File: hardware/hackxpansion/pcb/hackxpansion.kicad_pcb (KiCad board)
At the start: 4 copper layers, 52 x 69 mm, 101 parts, among them CN1 533981471, CN2 533981471, CN3 533981471, CN4 533981471, IC1 ADS7128IRTET, J1 Conn_01x03_MountingPin, J2 USB_C_Receptacle_USB2.0_14P, Q1 BSS138, Q2 2N7002, SW1 SW_Push, SW2 SW_Push, SW3 SW_On_Off, U2 RP2354B, U5 SPX3819M5-L-3-3, U7 BQ24075RGT, U8 USBLC6-2SC6, Y1 ABM8-272-T3

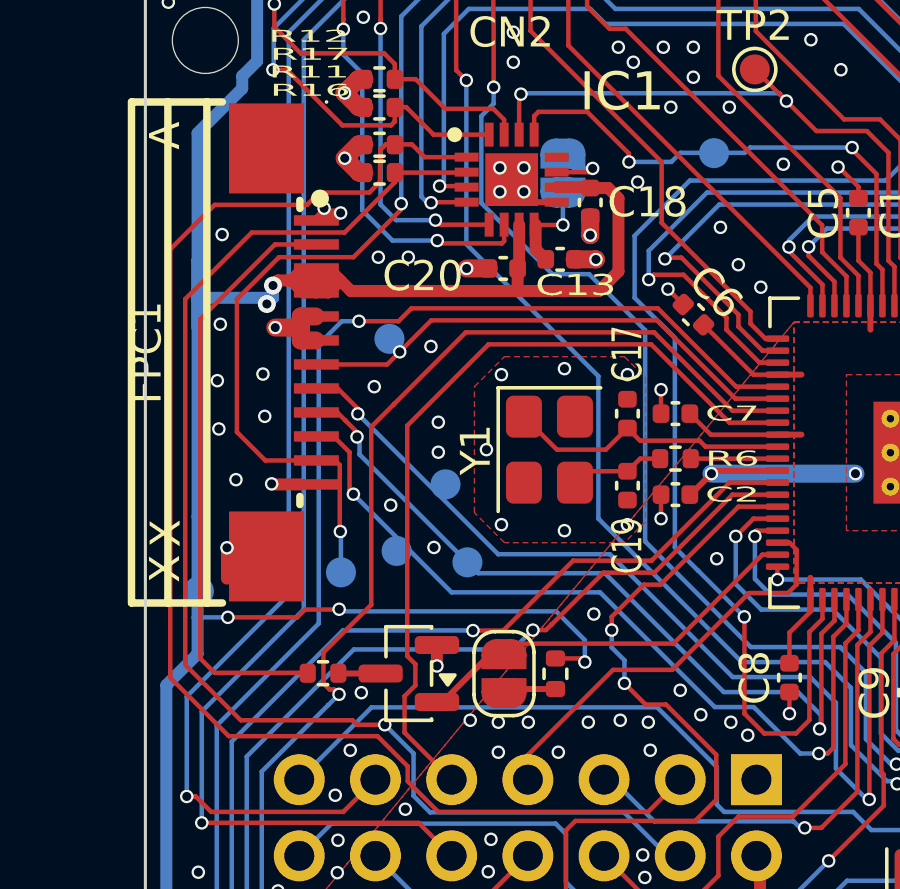
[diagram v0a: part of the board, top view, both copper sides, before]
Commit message: fixed issues with new fpc
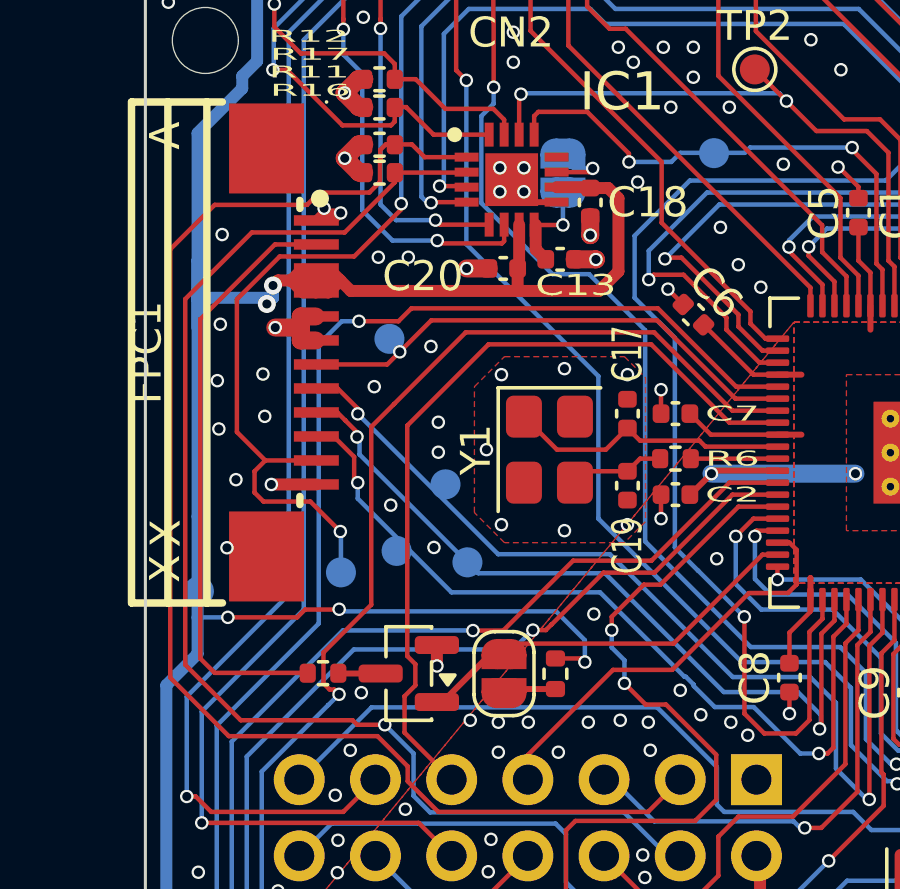
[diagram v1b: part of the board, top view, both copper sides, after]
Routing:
- net /GND: track 62.5 -> 64.4 mm
- net /Main Board/Display/RESET: track 59.8 -> 61.0 mm
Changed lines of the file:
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@@
 		(capping no)
 		(filling no)
-		(zone_defaults)
 		(grid_origin 122.239998 40.72)
 		(pcbplotparams
@@
 	)
 	(segment
+		(start 105.62 81.81)
+		(end 105.91 82.1)
+		(width 0.4)
+		(layer "F.Cu")
+		(net "/GND")
+	)
+	(segment
 		(start 147.610459 96.500266)
 		(end 148.149423 96.500266)
@@
 	)
 	(segment
+		(start 104.59 81.81)
+		(end 105.62 81.81)
+		(width 0.4)
+		(layer "F.Cu")
+		(net "/GND")
+	)
+	(segment
 		(start 114.83 70.29)
 		(end 114.08 69.54)
@@
 	)
 	(segment
-		(start 104.59 82.840001)
-		(end 104.59 81.81)
-		(width 0.4)
-		(layer "F.Cu")
-		(net "/GND")
-	)
-	(segment
 		(start 107.827121 70.622879)
 		(end 107.55 70.9)
@@
 	)
 	(segment
+		(start 107.57 79.7)
+		(end 106.069998 79.7)
+		(width 0.4)
+		(layer "F.Cu")
+		(net "/GND")
+	)
+	(segment
 		(start 127.244998 93.277787)
 		(end 127.244998 92.65)
@@
 	)
 	(via
+		(at 106.069998 79.7)
+		(size 0.45)
+		(drill 0.3)
+		(layers "F.Cu" "B.Cu")
+		(net "/GND")
+	)
+	(via
 		(at 136.2 97.06)
 		(size 0.45)
@@
 	)
 	(via
-		(at 106.08 79.68)
-		(size 0.45)
-		(drill 0.3)
-		(layers "F.Cu" "B.Cu")
-		(free yes)
-		(net "/GND")
-	)
-	(via
 		(at 103.635738 92.625706)
 		(size 0.45)
@@
 	)
 	(segment
-		(start 108.676572 79.89654)
-		(end 108.676572 78.626572)
-		(width 0.15)
-		(layer "F.Cu")
-		(net "/Main Board/Display/MOSI")
-	)
-	(segment
 		(start 124.32 88.668245)
 		(end 124.61 88.668245)
@@
 	)
 	(segment
-		(start 108.676572 78.626572)
+		(start 108.829998 78.779998)
 		(end 108.16 78.11)
 		(width 0.15)
@@
 	)
 	(segment
-		(start 107.559999 78.11)
-		(end 107.549999 78.1)
+		(start 108.829998 79.519995)
+		(end 108.829998 78.779998)
 		(width 0.15)
 		(layer "F.Cu")
@@
 	)
 	(segment
+		(start 107.559999 78.11)
+		(end 107.549999 78.1)
+		(width 0.15)
+		(layer "F.Cu")
+		(net "/Main Board/Display/MOSI")
+	)
+	(segment
 		(start 108.16 78.11)
 		(end 107.559999 78.11)
@@
 	)
 	(segment
-		(start 108.805016 80.024984)
-		(end 108.676572 79.89654)
+		(start 108.950003 79.64)
+		(end 108.829998 79.519995)
 		(width 0.15)
 		(layer "F.Cu")
@@
 	)
 	(via
-		(at 108.805016 80.024984)
+		(at 108.950003 79.64)
 		(size 0.45)
 		(drill 0.3)
@@
 	)
 	(segment
-		(start 120.85 87.12)
-		(end 122.15 87.12)
+		(start 122.15 87.12)
+		(end 123.698245 88.668245)
 		(width 0.15)
 		(layer "B.Cu")
@@
 	)
 	(segment
-		(start 112.075032 83.295)
-		(end 117.025 83.295)
+		(start 108.950003 80.169971)
+		(end 112.075032 83.295)
 		(width 0.15)
 		(layer "B.Cu")
@@
 	)
 	(segment
-		(start 122.15 87.12)
-		(end 123.698245 88.668245)
+		(start 108.950003 79.64)
+		(end 108.950003 80.169971)
 		(width 0.15)
 		(layer "B.Cu")
@@
 	)
 	(segment
-		(start 108.805016 80.024984)
-		(end 112.075032 83.295)
+		(start 120.85 87.12)
+		(end 122.15 87.12)
+		(width 0.15)
+		(layer "B.Cu")
+		(net "/Main Board/Display/MOSI")
+	)
+	(segment
+		(start 120.15 86.373603)
+		(end 120.15 86.42)
 		(width 0.15)
 		(layer "B.Cu")
@@
 	)
 	(segment
+		(start 119.886397 86.11)
+		(end 120.15 86.373603)
+		(width 0.15)
+		(layer "B.Cu")
+		(net "/Main Board/Display/MOSI")
+	)
+	(segment
 		(start 117.025 83.295)
+		(end 119.84 86.11)
+		(width 0.15)
+		(layer "B.Cu")
+		(net "/Main Board/Display/MOSI")
+	)
+	(segment
+		(start 119.84 86.11)
+		(end 119.886397 86.11)
+		(width 0.15)
+		(layer "B.Cu")
+		(net "/Main Board/Display/MOSI")
+	)
+	(segment
+		(start 120.15 86.42)
 		(end 120.85 87.12)
 		(width 0.15)
@@
 	)
 	(segment
-		(start 110.4 70.53)
-		(end 108.805 72.125)
+		(start 112.075032 83.295)
+		(end 117.025 83.295)
+		(width 0.15)
+		(layer "B.Cu")
+		(net "/Main Board/Display/MOSI")
+	)
+	(segment
+		(start 104.921117 77.951117)
+		(end 105.87 78.9)
 		(width 0.15)
 		(layer "F.Cu")
@@
 	)
 	(segment
-		(start 108.805 72.125)
-		(end 106.324999 72.125)
+		(start 107.37 80.27)
+		(end 105.809998 80.27)
 		(width 0.15)
 		(layer "F.Cu")
@@
 	)
 	(segment
-		(start 107.05 79.7)
-		(end 106.1 79.7)
-		(width 0.4)
+		(start 105.509998 79.97)
+		(end 105.509998 79.260002)
+		(width 0.15)
 		(layer "F.Cu")
 		(net "/Main Board/Display/RESET")
 	)
 	(segment
-		(start 131.890003 67.91)
-		(end 131.840001 67.960002)
+		(start 108.83 72.1)
+		(end 106.349999 72.1)
 		(width 0.15)
 		(layer "F.Cu")
@@
 	)
 	(segment
-		(start 105.87 78.9)
-		(end 107.05 78.9)
+		(start 105.509998 79.260002)
+		(end 105.87 78.9)
 		(width 0.15)
 		(layer "F.Cu")
@@
 	)
 	(segment
-		(start 131.840001 67.960002)
-		(end 131.840001 72.34)
+		(start 110.4 70.34)
+		(end 110.4 70.53)
 		(width 0.15)
 		(layer "F.Cu")
@@
 	)
 	(segment
-		(start 108.35 81.25)
-		(end 108.35 79.05)
+		(start 131.890003 67.91)
+		(end 131.840001 67.960002)
 		(width 0.15)
 		(layer "F.Cu")
@@
 	)
 	(segment
-		(start 104.921117 73.528882)
-		(end 104.921117 77.951117)
+		(start 105.87 78.9)
+		(end 107.05 78.9)
 		(width 0.15)
 		(layer "F.Cu")
@@
 	)
 	(segment
-		(start 108.35 79.05)
-		(end 108.2 78.9)
+		(start 131.840001 67.960002)
+		(end 131.840001 72.34)
 		(width 0.15)
 		(layer "F.Cu")
@@
 	)
 	(segment
-		(start 106.324999 72.125)
-		(end 104.921117 73.528882)
+		(start 105.809998 80.27)
+		(end 105.509998 79.97)
 		(width 0.15)
 		(layer "F.Cu")
@@
 	)
 	(segment
-		(start 131.840001 72.34)
-		(end 131.240001 72.94)
+		(start 106.349999 72.1)
+		(end 104.921117 73.528882)
 		(width 0.15)
 		(layer "F.Cu")
@@
 	)
 	(segment
-		(start 106.1 79.7)
-		(end 106.08 79.68)
+		(start 131.840001 72.34)
+		(end 131.240001 72.94)
 		(width 0.15)
 		(layer "F.Cu")
@@
 	)
 	(segment
-		(start 104.921117 77.951117)
-		(end 105.87 78.9)
+		(start 110.4 70.53)
+		(end 108.83 72.1)
 		(width 0.15)
 		(layer "F.Cu")
@@
 	)
 	(segment
-		(start 131.240001 72.94)
-		(end 131.240002 73.743499)
+		(start 108.37 81.27)
+		(end 107.37 80.27)
 		(width 0.15)
 		(layer "F.Cu")
@@
 	)
 	(segment
-		(start 107.8 78.9)
-		(end 107.05 78.9)
+		(start 104.921117 73.528882)
+		(end 104.921117 77.951117)
 		(width 0.15)
 		(layer "F.Cu")
@@
 	)
 	(segment
-		(start 108.37 81.27)
-		(end 108.35 81.25)
+		(start 131.240001 72.94)
+		(end 131.240002 73.743499)
 		(width 0.15)
 		(layer "F.Cu")
@@
 	)
 	(segment
-		(start 110.4 70.34)
-		(end 110.4 70.53)
+		(start 107.8 78.9)
+		(end 107.05 78.9)
 		(width 0.15)
 		(layer "F.Cu")
@@
 	)
 	(segment
-		(start 108.511644 71.301644)
-		(end 110.18677 69.626519)
+		(start 105.42 71.3)
+		(end 108.513289 71.3)
 		(width 0.15)
 		(layer "F.Cu")
@@
 	)
 	(segment
-		(start 103.2 85.710001)
-		(end 103.2 73.52)
+		(start 108.93 87.710001)
+		(end 108.78 87.560001)
 		(width 0.15)
 		(layer "F.Cu")
@@
 	)
 	(segment
-		(start 110.185591 69.304687)
-		(end 112.565313 69.304687)
+		(start 108.78 87.560001)
+		(end 105.05 87.560001)
 		(width 0.15)
 		(layer "F.Cu")
@@
 	)
 	(segment
-		(start 105.05 87.560001)
-		(end 103.2 85.710001)
+		(start 110.185591 69.304687)
+		(end 112.565313 69.304687)
 		(width 0.15)
 		(layer "F.Cu")
@@
 	)
 	(segment
-		(start 105.418356 71.301644)
-		(end 108.511644 71.301644)
+		(start 103.2 73.52)
+		(end 105.42 71.3)
 		(width 0.15)
 		(layer "F.Cu")
@@
 	)
 	(segment
-		(start 108.93 87.710001)
-		(end 108.78 87.560001)
+		(start 105.05 87.560001)
+		(end 103.2 85.710001)
 		(width 0.15)
 		(layer "F.Cu")
@@
 	)
 	(segment
-		(start 108.78 87.560001)
-		(end 105.05 87.560001)
+		(start 109.851316 87.71)
+		(end 109.851315 87.710001)
 		(width 0.15)
 		(layer "F.Cu")
@@
 	)
 	(segment
-		(start 109.851316 87.71)
-		(end 109.851315 87.710001)
+		(start 109.851315 87.710001)
+		(end 108.93 87.710001)
 		(width 0.15)
 		(layer "F.Cu")
@@
 	)
 	(segment
-		(start 103.2 73.52)
-		(end 105.418356 71.301644)
+		(start 103.2 85.710001)
+		(end 103.2 73.52)
 		(width 0.15)
 		(layer "F.Cu")
@@
 	)
 	(segment
-		(start 109.851315 87.710001)
-		(end 108.93 87.710001)
+		(start 108.513289 71.3)
+		(end 110.18677 69.626519)
 		(width 0.15)
 		(layer "F.Cu")
